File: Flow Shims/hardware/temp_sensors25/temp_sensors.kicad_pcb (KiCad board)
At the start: 2 copper layers, 6 x 113 mm, 52 parts, among them J1 Conn_01x03, U10 TMP1826NG, U11 TMP1826NG, U12 TMP1826NG, U13 TMP1826NG, U14 TMP1826NG, U15 TMP1826NG, U16 TMP1826NG, U17 TMP1826NG, U18 TMP1826NG, U19 TMP1826NG, U2 TMP1826NG, U20 TMP1826NG, U21 TMP1826NG, U22 TMP1826NG, U23 TMP1826NG, U24 TMP1826NG, U25 TMP1826NG, U26 TMP1826NG, U3 TMP1826NG, U4 TMP1826NG, U5 TMP1826NG, U6 TMP1826NG, U7 TMP1826NG, U8 TMP1826NG, U9 TMP1826NG

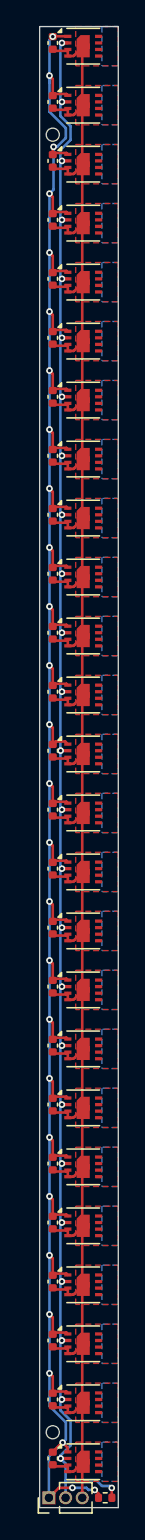
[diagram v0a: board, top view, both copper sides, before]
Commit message: Add firmware
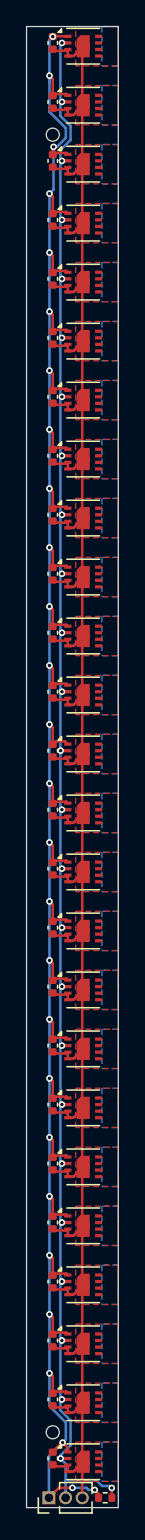
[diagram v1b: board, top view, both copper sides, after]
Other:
- board size 6 x 113 mm -> 7 x 113 mm
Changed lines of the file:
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@@
 		(capping no)
 		(filling no)
-		(zone_defaults)
 		(pcbplotparams
 			(layerselection 0x00000000_00000000_55555555_5755f5ff)
@@
 			(outputformat 1)
 			(mirror no)
-			(drillshape 1)
+			(drillshape 0)
 			(scaleselection 1)
-			(outputdirectory "")
+			(outputdirectory "cam/")
 		)
 	)
@@
 			(pinfunction "PAD_9")
 			(pintype "passive")
-			(zone_connect 0)
+			(zone_connect 2)
 			(options
 				(clearance outline)
@@
 			(pinfunction "PAD_9")
 			(pintype "passive")
-			(zone_connect 0)
+			(zone_connect 2)
 			(options
 				(clearance outline)
@@
 			(pinfunction "PAD_9")
 			(pintype "passive")
-			(zone_connect 0)
+			(zone_connect 2)
 			(options
 				(clearance outline)
@@
 			(pinfunction "PAD_9")
 			(pintype "passive")
-			(zone_connect 0)
+			(zone_connect 2)
 			(options
 				(clearance outline)
@@
 			(pinfunction "PAD_9")
 			(pintype "passive")
-			(zone_connect 0)
+			(zone_connect 2)
 			(options
 				(clearance outline)
@@
 			(pinfunction "PAD_9")
 			(pintype "passive")
-			(zone_connect 0)
+			(zone_connect 2)
 			(options
 				(clearance outline)
@@
 			(pinfunction "PAD_9")
 			(pintype "passive")
-			(zone_connect 0)
+			(zone_connect 2)
 			(options
 				(clearance outline)
@@
 			(pinfunction "PAD_9")
 			(pintype "passive")
-			(zone_connect 0)
+			(zone_connect 2)
 			(options
 				(clearance outline)
@@
 			(pinfunction "PAD_9")
 			(pintype "passive")
-			(zone_connect 0)
+			(zone_connect 2)
 			(options
 				(clearance outline)
@@
 			(pinfunction "PAD_9")
 			(pintype "passive")
-			(zone_connect 0)
+			(zone_connect 2)
 			(options
 				(clearance outline)
@@
 			(pinfunction "PAD_9")
 			(pintype "passive")
-			(zone_connect 0)
+			(zone_connect 2)
 			(options
 				(clearance outline)
@@
 			(pinfunction "PAD_9")
 			(pintype "passive")
-			(zone_connect 0)
+			(zone_connect 2)
 			(options
 				(clearance outline)
@@
 			(pinfunction "PAD_9")
 			(pintype "passive")
-			(zone_connect 0)
+			(zone_connect 2)
 			(options
 				(clearance outline)
@@
 			(pinfunction "PAD_9")
 			(pintype "passive")
-			(zone_connect 0)
+			(zone_connect 2)
 			(options
 				(clearance outline)
@@
 			(pinfunction "PAD_9")
 			(pintype "passive")
-			(zone_connect 0)
+			(zone_connect 2)
 			(options
 				(clearance outline)
@@
 			(pinfunction "PAD_9")
 			(pintype "passive")
-			(zone_connect 0)
+			(zone_connect 2)
 			(options
 				(clearance outline)
@@
 			(pinfunction "PAD_9")
 			(pintype "passive")
-			(zone_connect 0)
+			(zone_connect 2)
 			(options
 				(clearance outline)
@@
 			(pinfunction "PAD_9")
 			(pintype "passive")
-			(zone_connect 0)
+			(zone_connect 2)
 			(options
 				(clearance outline)
@@
 			(pinfunction "PAD_9")
 			(pintype "passive")
-			(zone_connect 0)
+			(zone_connect 2)
 			(options
 				(clearance outline)
@@
 			(pinfunction "PAD_9")
 			(pintype "passive")
-			(zone_connect 0)
+			(zone_connect 2)
 			(options
 				(clearance outline)
@@
 			(pinfunction "PAD_9")
 			(pintype "passive")
-			(zone_connect 0)
+			(zone_connect 2)
 			(options
 				(clearance outline)
@@
 			(pinfunction "PAD_9")
 			(pintype "passive")
-			(zone_connect 0)
+			(zone_connect 2)
 			(options
 				(clearance outline)
@@
 			(pinfunction "PAD_9")
 			(pintype "passive")
-			(zone_connect 0)
+			(zone_connect 2)
 			(options
 				(clearance outline)
@@
 			(pinfunction "PAD_9")
 			(pintype "passive")
-			(zone_connect 0)
+			(zone_connect 2)
 			(options
 				(clearance outline)
@@
 			(pinfunction "PAD_9")
 			(pintype "passive")
-			(zone_connect 0)
+			(zone_connect 2)
 			(options
 				(clearance outline)
@@
 	)
 	(gr_rect
-		(start 139 44.75)
+		(start 138 44.75)
 		(end 145 157.75)
 		(stroke
